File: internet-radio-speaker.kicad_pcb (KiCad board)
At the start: 4 copper layers, 60 x 44 mm, 73 parts, among them IC301 MAX98357AETE+T, IC302 MAX98357AETE+T, J1 USB-TYPE-C-018, J2 BAT_CON, J201 WIFI_ANT, J301 L_SPKR, J302 R_SPKR, Q1 DMP1045U-7, SW201 BOOT_SEL, U1 USBLC6-2SC6, U101 LP4054H, U201 ESP32C3, U202 W25Q32JVSS, U4 XC9141, U8 TPS63000, Y201 40MHz

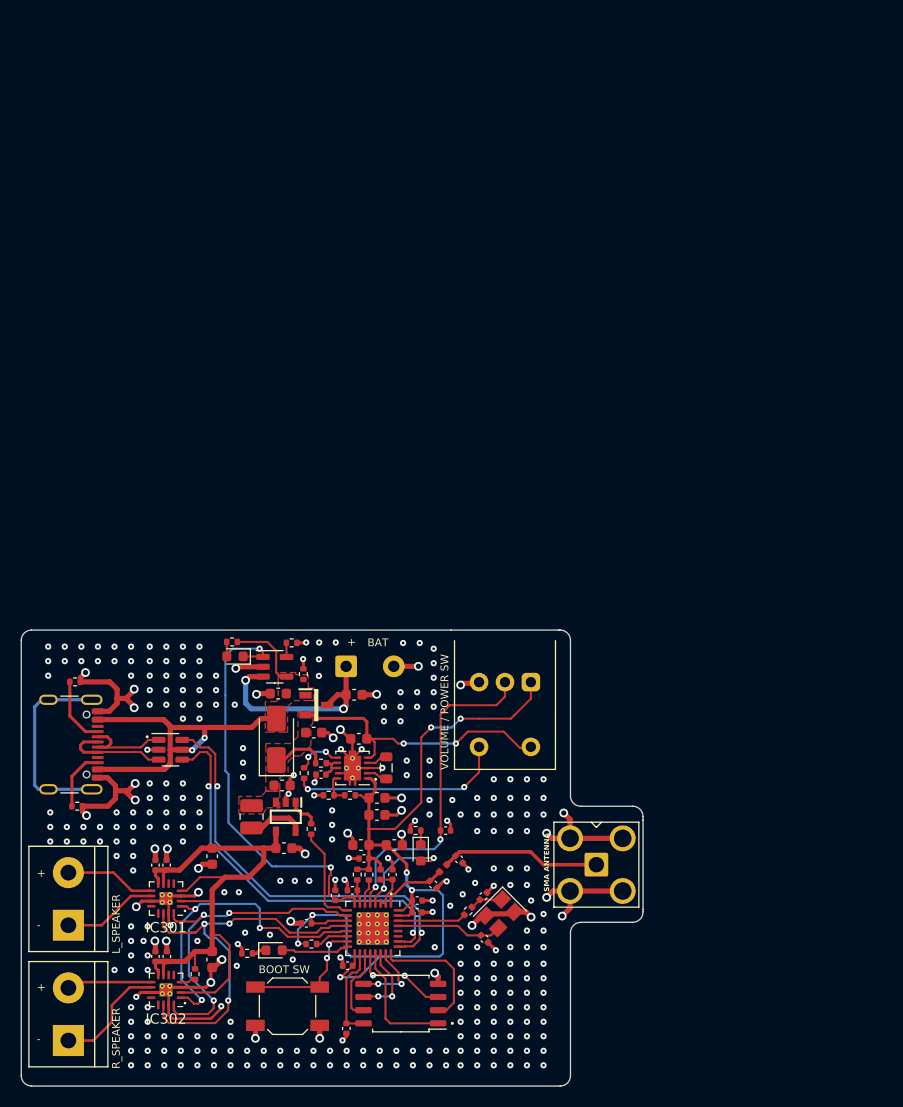
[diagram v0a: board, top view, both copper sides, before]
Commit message: updated to rev 3
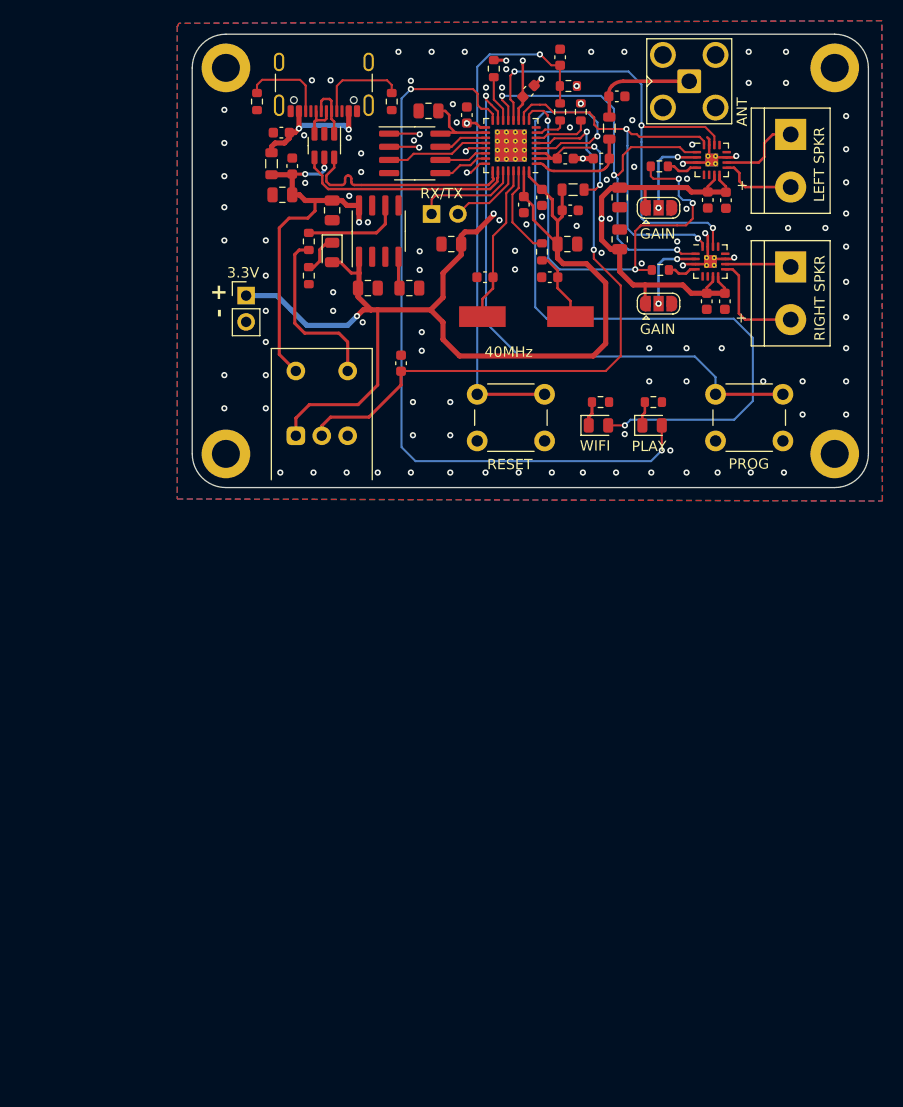
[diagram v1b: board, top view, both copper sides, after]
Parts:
- removed C1, C10, C3, C306, C4, C5, C7, C8, C9: 10u, Capacitor_SMD:C_0603_1608Metric
- removed C2, C213, C6: 100n, Capacitor_SMD:C_0402_1005Metric
- removed D1: CHR_LED, LED_SMD:LED_0603_1608Metric
- removed D2: SS14, Diode_SMD:D_SMA
- removed J2: BAT_CON, Connector_Wire:SolderWire-0.5sqmm_1x02_P4.6mm_D0.9mm_OD2.1mm
- removed L1: 2u2, Inductor_SMD:L_0805_2012Metric
- removed L2: 4u7, Inductor_SMD:L_1008_2520Metric
- removed Q1: DMP1045U-7, Internet_Radio_Speaker:SOT96P240X120-3N
- removed R10, R6, R7: 100, Resistor_SMD:R_0402_1005Metric
- removed R3, R4: 2k, Resistor_SMD:R_0402_1005Metric
- removed R5: 100k, Resistor_SMD:R_0402_1005Metric
- removed R8: 1M, Resistor_SMD:R_0402_1005Metric
- removed R9: 200k, Resistor_SMD:R_0402_1005Metric
- removed U4: XC9141, Internet_Radio_Speaker:SOT95P280X130-5N
- removed U8: TPS63000, Package_SON:Texas_DRC0010J_ThermalVias
- removed Y201: 40MHz, Crystal:Crystal_SMD_3225-4Pin_3.2x2.5mm
- added C101: 10u, Capacitor_SMD:C_0805_2012Metric, F.Cu at (141.4, 57.0)
- added C102: DNP, Capacitor_SMD:C_0805_2012Metric, F.Cu at (145.4, 57.0)
- added C103: 10n, Capacitor_SMD:C_0603_1608Metric, F.Cu at (133.1, 42.0)
- added C104: 100n, Capacitor_SMD:C_0603_1608Metric, F.Cu at (134.2, 45.2)
- added C105: 10u, Capacitor_SMD:C_0805_2012Metric, F.Cu at (138.0, 49.5)
- added C107: 10u, Capacitor_SMD:C_0805_2012Metric, F.Cu at (133.2, 48.0)
- added C216: 10u, Capacitor_SMD:C_0805_2012Metric, F.Cu at (160.7, 52.8)
- added C307: 10u, Capacitor_SMD:C_0805_2012Metric, F.Cu at (165.8, 48.2)
- added D101: PWR_LED, LED_SMD:LED_0805_2012Metric, F.Cu at (138.0, 53.6)
- added H101: MountingHole_Pad, MountingHole:MountingHole_2.7mm_M2.5_DIN965_Pad, F.Cu at (127.8, 35.8)
- added H102: MountingHole_Pad, MountingHole:MountingHole_2.7mm_M2.5_DIN965_Pad, F.Cu at (186.5, 35.8)
- added H103: MountingHole_Pad, MountingHole:MountingHole_2.7mm_M2.5_DIN965_Pad, F.Cu at (127.8, 73.0)
- added H104: MountingHole_Pad, MountingHole:MountingHole_2.7mm_M2.5_DIN965_Pad, F.Cu at (186.5, 73.0)
- added J202: UART, Connector_PinSocket_2.54mm:PinSocket_1x02_P2.54mm_Vertical, B.Cu at (147.6, 49.9)
- added J203: EXT_PWR, Connector_PinHeader_2.54mm:PinHeader_1x02_P2.54mm_Vertical, F.Cu at (129.7, 57.7)
- added JP301: GAIN, Jumper:SolderJumper-3_P1.3mm_Open_RoundedPad1.0x1.5mm, F.Cu at (169.5, 58.5)
- added JP305: GAIN, Jumper:SolderJumper-3_P1.3mm_Open_RoundedPad1.0x1.5mm, F.Cu at (169.5, 49.3)
- added L203: 3u3, Inductor_SMD:L_0805_2012Metric, F.Cu at (132.2, 45.0)
- added R101: 10k, Resistor_SMD:R_0603_1608Metric, F.Cu at (135.8, 52.5)
- added R102: 5k1, Resistor_SMD:R_0603_1608Metric, F.Cu at (135.8, 55.8)
- added R207: 22, Resistor_SMD:R_0603_1608Metric, F.Cu at (160.0, 40.0)
- added R302: 0, Resistor_SMD:R_0603_1608Metric, F.Cu at (169.6, 45.2)
- added SW202: RST_SW, Button_Switch_THT:SW_PUSH_6mm, F.Cu at (158.5, 71.8)
- added Y202: 40MHz, Crystal:Crystal_SMD_HC49-SD, F.Cu at (156.8, 59.8)
- C201, C203, C204, C205, C206, C207, C209, C210, C211, C212, C214, C215, C301, C302, C304, C305: footprint Capacitor_SMD:C_0402_1005Metric -> Capacitor_SMD:C_0603_1608Metric
- C202, C208, C303: footprint Capacitor_SMD:C_0603_1608Metric -> Capacitor_SMD:C_0805_2012Metric
- D201, D202: footprint LED_SMD:LED_0603_1608Metric -> LED_SMD:LED_0805_2012Metric
- J1: value USB-TYPE-C-018 -> USB_C_Receptacle_USB2.0
- L201, L202: footprint Inductor_SMD:L_0402_1005Metric -> Inductor_SMD:L_0805_2012Metric
- R1, R2, R203, R206, R301: footprint Resistor_SMD:R_0402_1005Metric -> Resistor_SMD:R_0603_1608Metric
- R201, R204, R205: value 10k -> 5k1; footprint Resistor_SMD:R_0402_1005Metric -> Resistor_SMD:R_0603_1608Metric
- R202: value 100 -> 22; footprint Resistor_SMD:R_0402_1005Metric -> Resistor_SMD:R_0603_1608Metric
- SW201: footprint Button_Switch_SMD:SW_SPST_SKQG_WithoutStem -> Button_Switch_THT:SW_PUSH_6mm
- U101: value LP4054H -> TC1263; footprint Package_TO_SOT_SMD:SOT-23-5 -> Package_SO:SOIC-8_3.9x4.9mm_P1.27mm
- U202: footprint Package_SO:SOIC-8_5.23x5.23mm_P1.27mm -> Package_SO:SOIC-8_3.9x4.9mm_P1.27mm
- moved J301 103.4 mm to (182.2, 42.2), turned to -90 degrees
- moved J302 102.1 mm to (182.2, 55.0), turned to -90 degrees
- moved IC301 88.6 mm to (174.6, 44.6), turned to 0 degrees
- moved IC302 87.7 mm to (174.5, 54.4), turned to 0 degrees
- moved R205 86.3 mm to (153.6, 35.8), turned to 90 degrees
- moved C302 83.8 mm to (176.0, 48.5), turned to -90 degrees
- moved C305 83.8 mm to (175.9, 58.3), turned to -90 degrees
- moved C301 83.4 mm to (174.2, 48.5), turned to -90 degrees
- moved C206 83.1 mm to (156.9, 38.0), turned to 45 degrees
- moved C205 82.9 mm to (151.0, 40.3), turned to 90 degrees
- moved C201 82.9 mm to (160.0, 34.7), turned to 90 degrees
- moved U202 82.1 mm to (146.0, 44.0), turned to 0 degrees
- moved C304 81.9 mm to (174.2, 58.3), turned to -90 degrees
- moved R301 81.4 mm to (169.7, 55.2), turned to 0 degrees
- moved R201 78.8 mm to (160.8, 37.5), turned to 180 degrees
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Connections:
- net /CC1 renamed Net-(J1-CC1)
- net /CC2 renamed Net-(J1-CC2)
- net /mcu/D_CAP renamed /Microcontroller/3V3
- net /mcu/PCB_ANTENNA renamed /Microcontroller/PCB_ANTENNA
- net /mcu/PLAYING_LED renamed /Microcontroller/PLAYING_LED
- net /mcu/PU_GPIO2 renamed /Microcontroller/PU_GPIO2
- net /mcu/PU_GPIO8 renamed /Microcontroller/PU_GPIO8
- net /mcu/RF_ANTENNA renamed /Microcontroller/RF_ANTENNA
- net /mcu/SPICS0 renamed /Microcontroller/SPICS0
- net /mcu/SPICSLK renamed /Microcontroller/SPICSLK
- net /mcu/SPID renamed /Microcontroller/SPID
- net /mcu/SPIHD renamed /Microcontroller/SPIHD
- net /mcu/SPIQ renamed /Microcontroller/SPIQ
- net /mcu/SPIWP renamed /Microcontroller/SPIWP
- net /mcu/VR_VOL_CONTROL renamed /Microcontroller/VR_VOL_CONTROL
- net /mcu/WIFI_CUR_R renamed /Microcontroller/WIFI_CUR_R
- net /mcu/WIFI_LED renamed /Microcontroller/WIFI_LED
- net /mcu/XTAL_N renamed /Microcontroller/XTAL_N
- net I2SO_BCK_OUT renamed /Amplifiers/I2S0_BCK_IN
- net I2SO_SD_OUT renamed /Amplifiers/I2S0_SD_IN
- net I2SO_WS_OUT renamed /Amplifiers/I2S0_WS_IN
- C201 pad 1: /mcu/CHIP_EN -> /Microcontroller/CHIP_EN
- C208 pad 1: +3V3 -> /Microcontroller/VDD_SPI
- C211 pad 1: /mcu/XTAL_P -> /Microcontroller/XTAL_P
- IC301 pad 2: +5V -> Net-(IC301-GAIN)
- IC301 pad 4: +5V -> Net-(IC301-~{SD_MODE})
- IC302 pad 2: +5V -> Net-(IC302-GAIN)
- R201 pad 2: /mcu/CHIP_EN -> /Microcontroller/CHIP_EN
- R202 pad 1: /mcu/LIMIT_R -> /Microcontroller/XTAL_P
- R202 pad 2: /mcu/XTAL_P -> /Microcontroller/XTAL_L
- R301 pad 1: +5V -> /Amplifiers/AMP_SW
- U1 pad 5: VBUS -> +5V
- U101 pad 1: /mcu/BAT_STAT -> +3V3
- U101 pad 3: /BAT_CON_P -> unconnected-(U101-NC-Pad3)
- U101 pad 4: VBUS -> Net-(U101-BYPASS)
- U101 pad 5: /ISET -> unconnected-(U101-ERROR-Pad5)
- U201 pad 18: /mcu/VDD_SPI -> /Microcontroller/VDD_SPI
- U201 pad 27: unconnected-(U201-U0RXD/IO-Pad27) -> Net-(J202-Pin_1)
- U201 pad 28: unconnected-(U201-U0TXD/IO-Pad28) -> Net-(J202-Pin_2)
- U201 pad 30: /mcu/LIMIT_R -> /Microcontroller/XTAL_L
- U201 pad 7: /mcu/CHIP_EN -> Net-(U201-CHIP_EN)
- U201 pad 8: /mcu/BAT_STAT -> unconnected-(U201-GPIO3/ANALOG-Pad8)
- U201 pad 9: /AMP_SW -> /Amplifiers/AMP_SW
- U202 pad 8: /mcu/VDD_SPI -> /Microcontroller/VDD_SPI
- VR1 pad 4: VCC -> +5V
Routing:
- net GND: track 146.3 -> 16.4 mm, vias 326 -> 112
- net /Microcontroller/PLAYING_LED: track 6.56 -> 73.6 mm, vias 0 -> 2
- net /Microcontroller/WIFI_LED: track 9.98 -> 75.7 mm
- net +3V3: track 94.1 -> 152.9 mm
- net /Microcontroller/CHIP_EN: track 0.00 -> 50.7 mm, vias 0 -> 1
- net +5V: track 59.0 -> 105.0 mm, vias 0 -> 4
- net /Amplifiers/AMP_SW: track 0.00 -> 45.3 mm, vias 0 -> 4
- net Net-(SW201-A): track 12.6 -> 57.2 mm, vias 2 -> 1
- net /mcu/BAT_STAT: track 40.3 -> 0.00 mm, vias 2 -> 0
- net VCC: track 33.2 -> 0.00 mm, vias 2 -> 0
- net /Microcontroller/VR_VOL_CONTROL: track 32.0 -> 61.8 mm
- net VBUS: track 41.9 -> 12.8 mm
- net /BAT_CON_P: track 20.1 -> 0.00 mm, vias 2 -> 0
- net USB_D-: track 40.2 -> 21.2 mm, vias 2 -> 0
- net USB_D+: track 38.7 -> 21.3 mm, vias 2 -> 0
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- added copper zone on B.Cu, net GND
- added copper zone on F.Cu, net GND
- removed copper zone on F.Cu, net VBUS
- removed copper zone on F.Cu, net VCC
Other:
- board size 60 x 44 mm -> 65.2 x 43.8 mm
- board text added: "+ -"
- board text added: "3.3V"
- board text added: "40MHz"
- board text added: "ANT"
- board text added: "GAIN"
- board text added: "LEFT SPKR"
- board text added: "PLAY"
- board text added: "PROG"
- board text added: "RESET"
- board text added: "RIGHT SPKR"
- board text added: "RX/TX"
- board text added: "WIFI"
- board text removed: "-"
- board text removed: "BAT"
- board text removed: "BOOT SW"
- board text removed: "L_SPEAKER"
- board text removed: "R_SPEAKER"
- board text removed: "SMA ANTENNA"
- board text removed: "VOLUME / POWER SW"

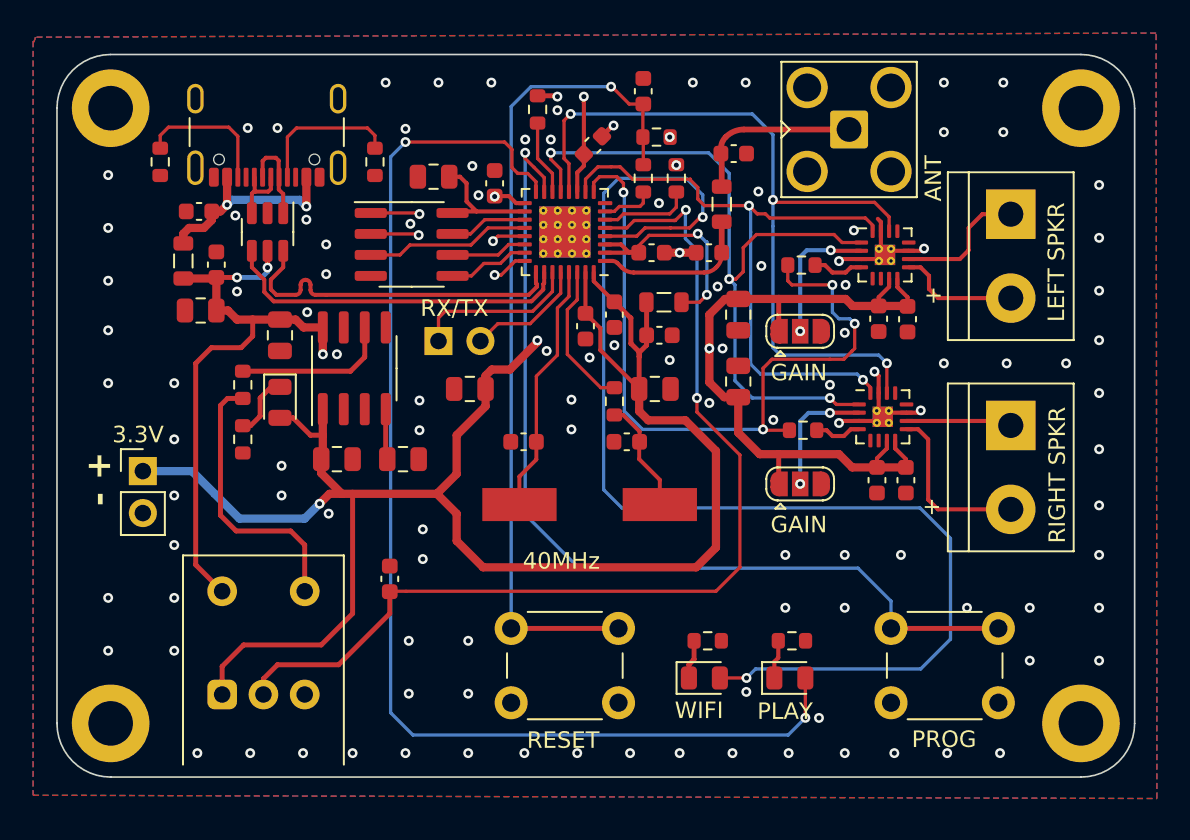
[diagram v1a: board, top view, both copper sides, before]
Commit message: updated to rev 4
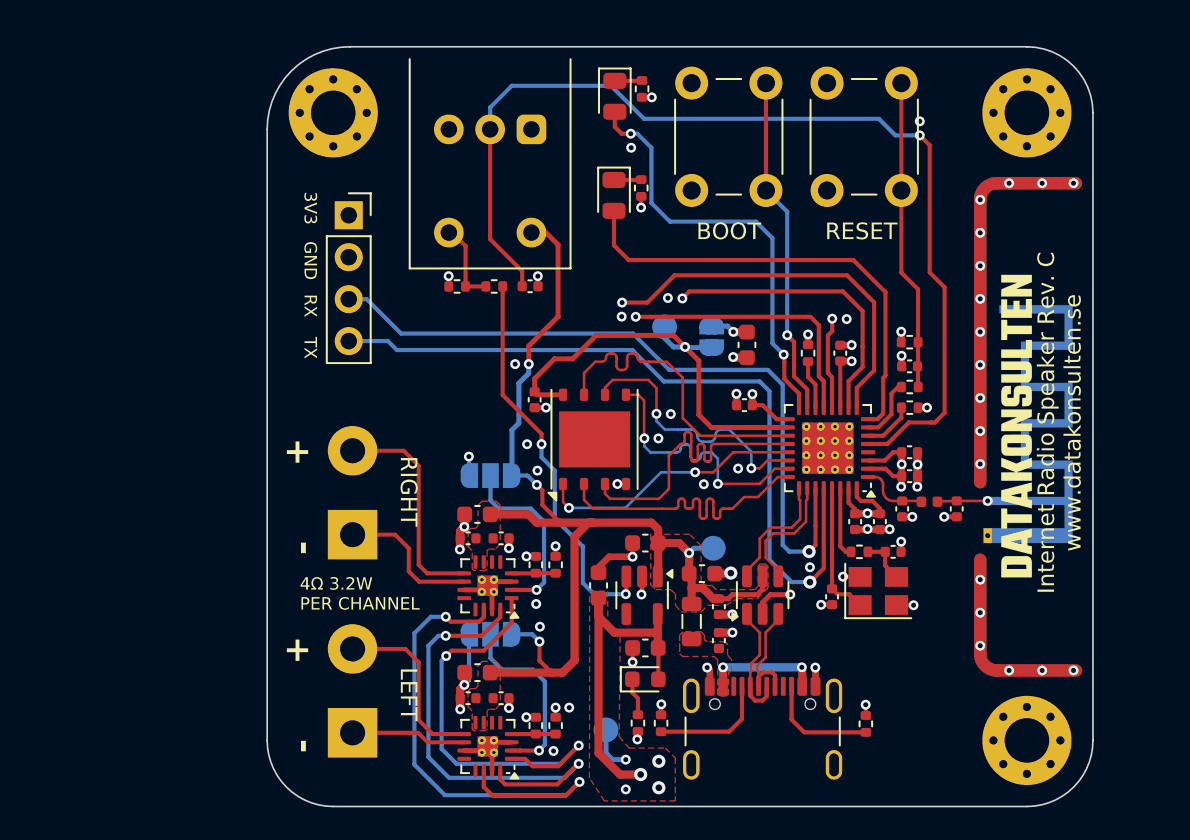
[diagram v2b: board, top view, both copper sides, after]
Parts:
- removed C102: DNP, Capacitor_SMD:C_0805_2012Metric
- removed H101: MountingHole_Pad, MountingHole:MountingHole_2.7mm_M2.5_DIN965_Pad
- removed J203: EXT_PWR, Connector_PinHeader_2.54mm:PinHeader_1x02_P2.54mm_Vertical
- removed L201: 2n2, Inductor_SMD:L_0805_2012Metric
- removed L203: 3u3, Inductor_SMD:L_0805_2012Metric
- removed U101: TC1263, Package_SO:SOIC-8_3.9x4.9mm_P1.27mm
- removed Y202: 40MHz, Crystal:Crystal_SMD_HC49-SD
- added FB101: BLM21SP601SN1D, Inductor_SMD:L_0805_2012Metric, F.Cu at (162.9, 66.8)
- added G***: LOGO, LOGO, F.Cu at (182.6, 55.0)
- added JP201: EXT_3V3, Jumper:SolderJumper-2_P1.3mm_Open_RoundedPad1.0x1.5mm, B.Cu at (164.1, 49.6)
- added R103: 1k, Resistor_SMD:R_0402_1005Metric, F.Cu at (151.0, 46.5)
- added R303: 100k, Resistor_SMD:R_0402_1005Metric, F.Cu at (153.5, 73.1)
- added R304: 100k, Resistor_SMD:R_0402_1005Metric, F.Cu at (153.5, 63.4)
- added TP101: 5V_TP, TestPoint:TestPoint_Pad_D1.5mm, B.Cu at (164.2, 62.4)
- added TP102: 3V3_TP, TestPoint:TestPoint_Pad_D1.5mm, B.Cu at (157.7, 73.4)
- added TP201: VDD_SPI_TP, TestPoint:TestPoint_Pad_D1.5mm, B.Cu at (161.3, 49.0)
- added U102: AP2112K-3.3, Package_TO_SOT_SMD:SOT-23-5, F.Cu at (159.9, 65.2)
- added Y201: 40MHz 10p5, Crystal:Crystal_SMD_3225-4Pin_3.2x2.5mm, F.Cu at (174.2, 65.0)
- C101, C105, C107, C202, C216, C303, C307: footprint Capacitor_SMD:C_0805_2012Metric -> Capacitor_SMD:C_0603_1608Metric
- C103, C104, C201, C203, C204, C205, C206, C207, C214, C215, C301, C302, C304, C305: footprint Capacitor_SMD:C_0603_1608Metric -> Capacitor_SMD:C_0402_1005Metric
- C208: value 10u -> 100n; footprint Capacitor_SMD:C_0805_2012Metric -> Capacitor_SMD:C_0402_1005Metric
- C209, C210: value 3p3 -> 1p8; footprint Capacitor_SMD:C_0603_1608Metric -> Capacitor_SMD:C_0402_1005Metric
- C211, C212: value 10p -> 12p; footprint Capacitor_SMD:C_0603_1608Metric -> Capacitor_SMD:C_0402_1005Metric
- D101: footprint LED_SMD:LED_0805_2012Metric -> LED_SMD:LED_0603_1608Metric
- H102, H103, H104: footprint MountingHole:MountingHole_2.7mm_M2.5_DIN965_Pad -> MountingHole:MountingHole_2.7mm_M2.5_Pad_Via
- J201: footprint Connector_Coaxial:SMA_Amphenol_901-143_Horizontal -> Internet_Radio_Speaker:Texas_SWRA117D_2.4GHz_Right; moved to B.Cu
- J202: value UART -> Conn_01x04; footprint Connector_PinSocket_2.54mm:PinSocket_1x02_P2.54mm_Vertical -> Connector_PinSocket_2.54mm:PinSocket_1x04_P2.54mm_Vertical; moved to F.Cu
- JP301, JP305: moved to B.Cu
- L202: value 2n2 -> 2n7; footprint Inductor_SMD:L_0805_2012Metric -> Inductor_SMD:L_0402_1005Metric
- R1, R2, R201, R204, R205, R301, R302: footprint Resistor_SMD:R_0603_1608Metric -> Resistor_SMD:R_0402_1005Metric
- R101: value 10k -> 5k1; footprint Resistor_SMD:R_0603_1608Metric -> Resistor_SMD:R_0402_1005Metric
- R102, R203, R206: value 5k1 -> 1k; footprint Resistor_SMD:R_0603_1608Metric -> Resistor_SMD:R_0402_1005Metric
- R202, R207: value 22 -> 22R; footprint Resistor_SMD:R_0603_1608Metric -> Resistor_SMD:R_0402_1005Metric
- U202: value W25Q32JVSS -> W25Q128JVPIQ; footprint Package_SO:SOIC-8_3.9x4.9mm_P1.27mm -> Package_SON:WSON-8-1EP_6x5mm_P1.27mm_EP3.4x4.3mm
- moved H103 55.5 mm to (183.2, 74.0), turned to 90 degrees
- moved R2 54.6 mm to (173.5, 73.0), turned to 90 degrees
- moved J301 50.7 mm to (142.4, 73.6), turned to 90 degrees
- moved J1 48.6 mm to (167.2, 74.4), turned to 0 degrees
- moved H102 45.3 mm to (141.2, 36.0), turned to 90 degrees
- moved C103 40.8 mm to (164.6, 68.0), turned to 90 degrees
- moved J302 40.4 mm to (142.4, 61.6), turned to 90 degrees
- moved IC301 38.3 mm to (150.6, 74.4), turned to 180 degrees
- moved R1 38.2 mm to (161.1, 73.0), turned to 90 degrees
- moved U1 37.2 mm to (167.2, 65.2), turned to 90 degrees
- moved H104 37.1 mm to (183.2, 36.0), turned to 90 degrees
- moved C104 36.8 mm to (164.6, 65.9), turned to -90 degrees
- moved D202 36.8 mm to (158.3, 35.0), turned to -90 degrees
- moved C302 35.1 mm to (149.4, 71.5), turned to 180 degrees
- moved R206 34.6 mm to (159.9, 34.6), turned to -90 degrees
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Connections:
- net /Microcontroller/WIFI_CUR_R renamed Net-(D201-K)
- C204 pad 1: /Microcontroller/3V3 -> +3V3
- C211 pad 1: /Microcontroller/XTAL_P -> GND
- C211 pad 2: GND -> /Microcontroller/XTAL_N
- C212 pad 1: /Microcontroller/XTAL_N -> GND
- C212 pad 2: GND -> /Microcontroller/XTAL_P
- J202 pad 1: Net-(J202-Pin_1) -> +3V3
- J202 pad 2: Net-(J202-Pin_2) -> GND
- R101 pad 1: Net-(U101-SHDN) -> /VR_PWR
- R101 pad 2: /VR_PWR -> GND
- R201 pad 1: +3V3 -> /Microcontroller/CHIP_EN
- R201 pad 2: /Microcontroller/CHIP_EN -> +3V3
- R206 pad 1: GND -> Net-(D202-K)
- R206 pad 2: Net-(D202-K) -> GND
- SW201 pad 1: Net-(SW201-A) -> GND
- SW201 pad 2: GND -> /Microcontroller/BOOT_SEL
- U201 pad 15: Net-(SW201-A) -> /Microcontroller/BOOT_SEL
- U201 pad 2: /Microcontroller/3V3 -> +3V3
- U201 pad 27: Net-(J202-Pin_1) -> /Microcontroller/UART_RX
- U201 pad 28: Net-(J202-Pin_2) -> /Microcontroller/UART_TX
- U201 pad 3: /Microcontroller/3V3 -> +3V3
- U201 pad 4: /Microcontroller/WIFI_LED -> unconnected-(U201-XTAL_32K_P/IO/ANALOG-Pad4)
- U201 pad 8: unconnected-(U201-GPIO3/ANALOG-Pad8) -> /Microcontroller/WIFI_LED
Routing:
- net +3V3: track 152.9 -> 47.4 mm, vias 7 -> 14
- net GND: track 16.4 -> 119.3 mm, vias 112 -> 76
- net Net-(SW201-A): track 57.2 -> 0.00 mm, vias 1 -> 0
- net /Microcontroller/WIFI_LED: track 75.7 -> 28.2 mm, vias 2 -> 0
- net /Microcontroller/PLAYING_LED: track 73.6 -> 26.1 mm
- net /Microcontroller/UART_TX: track 0.00 -> 46.0 mm, vias 0 -> 1
- net /Microcontroller/UART_RX: track 0.00 -> 43.9 mm, vias 0 -> 1
- net +5V: track 105.0 -> 66.2 mm
- net /Amplifiers/I2S0_BCK_IN: track 38.5 -> 76.8 mm, vias 2 -> 3
- net /Microcontroller/CHIP_EN: track 50.7 -> 18.8 mm, vias 1 -> 0
- net /Amplifiers/I2S0_WS_IN: track 48.1 -> 77.4 mm
- net unconnected-(J1-SHIELD-PadS1)_2: track 28.4 -> 0.00 mm
- net /Amplifiers/I2S0_SD_IN: track 44.9 -> 69.7 mm
- net /EN: track 0.00 -> 23.9 mm, vias 0 -> 2
- net /Microcontroller/BOOT_SEL: track 0.00 -> 20.7 mm, vias 0 -> 1
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- added copper zone on F.Cu, net +3V3
- added copper zone on In2.Cu, net +3V3
- added copper zone on F.Cu, net +5V
- added copper zone on F.Cu, net VBUS
- removed copper zone on B.Cu, net GND
- removed copper zone on F.Cu, net GND
- removed copper zone on In2.Cu, net GND
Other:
- board size 65.2 x 43.8 mm -> 50 x 46 mm
- board text added: "+3V3"
- board text added: "+5V"
- board text added: "-"
- board text added: "3V3"
- board text added: "4Ω 3.2W PER CHANNEL"
- board text added: "BOOT"
- board text added: "EXT_3V3_SPI"
- board text added: "GAIN_L"
- board text added: "GAIN_R"
- board text added: "GND"
- board text added: "Internet Radio Speaker Rev. C www.datakonsulten.se"
- board text added: "LEFT"
- board text added: "RIGHT"
- board text added: "RX"
- board text added: "TX"
- board text removed: "+ -"
- board text removed: "3.3V"
- board text removed: "40MHz"
- board text removed: "ANT"
- board text removed: "GAIN"
- board text removed: "LEFT SPKR"
- board text removed: "PLAY"
- board text removed: "PROG"
- board text removed: "RIGHT SPKR"
- board text removed: "RX/TX"
- board text removed: "WIFI"
